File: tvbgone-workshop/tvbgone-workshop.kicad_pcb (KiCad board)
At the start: 2 copper layers, 66.1 x 56 mm, 29 parts, among them IC1 ATTINY85-S, Q1 MOSFET_N, Q2 MOSFET_N, SW1 SW_PUSH_SMALL, X1 8MHz

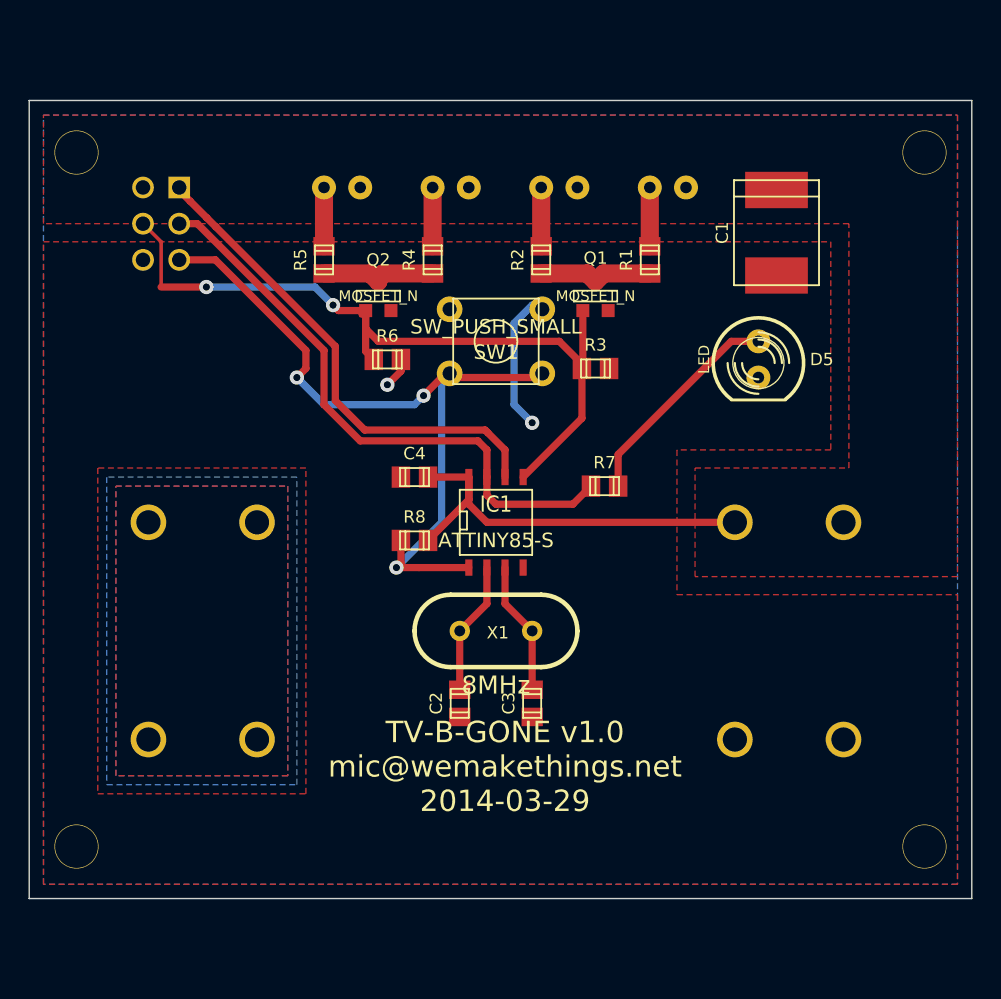
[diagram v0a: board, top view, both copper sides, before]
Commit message: opit
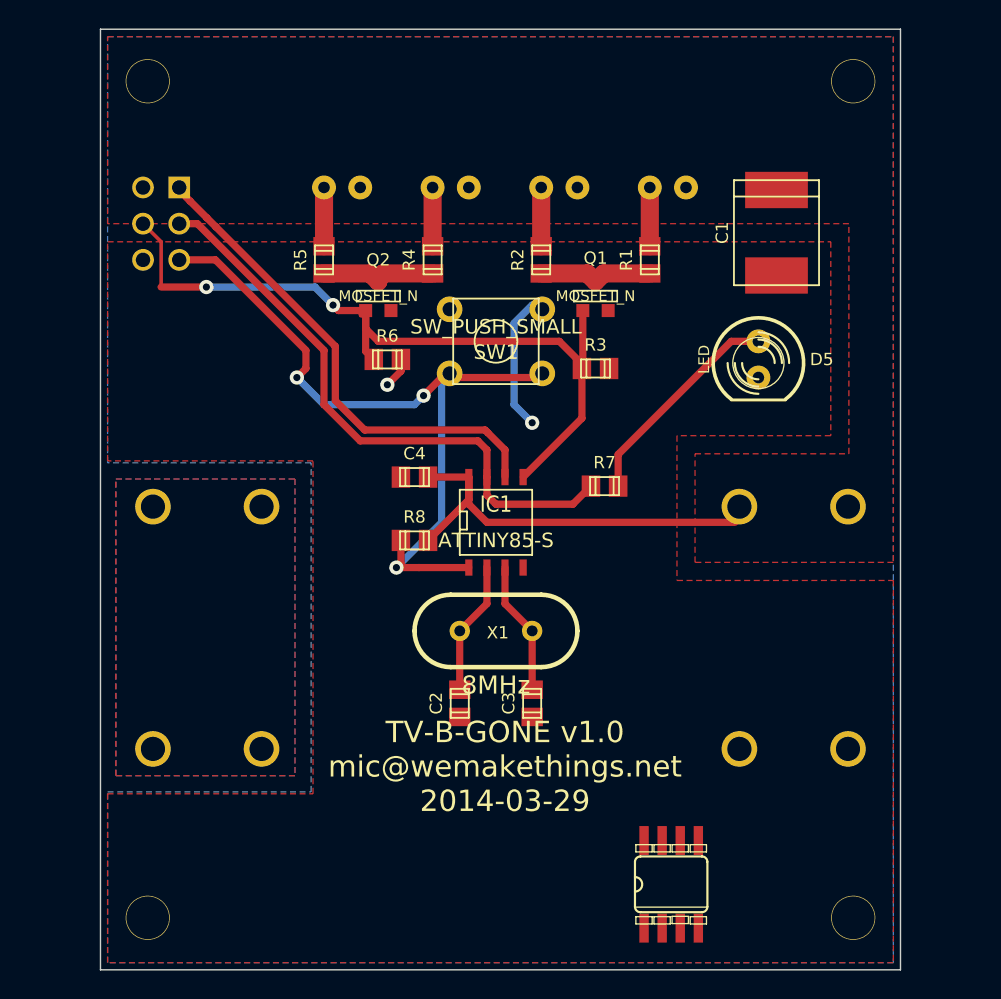
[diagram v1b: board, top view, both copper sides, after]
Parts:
- added >VALUE: >NAME, dallas-SOIC-8, F.Cu at (128.5, 127.0)
- moved BT1 1.14 mm to (117.2, 100.5)
- moved BT2 0.73 mm to (117.2, 117.5)
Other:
- board size 66.1 x 56 mm -> 56.1 x 66 mm
